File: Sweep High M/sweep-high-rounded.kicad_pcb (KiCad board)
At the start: 2 copper layers, 114.5 x 95.3 mm, 25 parts, among them J2 AudioJack4dpb, SW10 SW_Push, SW11 SW_Push, SW12 SW_Push, SW14 SW_Push, SW15 SW_Push, SW16 SW_Push, SW17 SW_Push, SW18 SW_Push, SW2 SW_Push, SW2 SW_SPDT, SW20 SW_Push, SW21 SW_Push, SW3 SW_Push, SW4 SW_Push, SW5 SW_Push, SW6 SW_Push, SW8 SW_Push, SW9 SW_Push, U1 ProMicro-kbd

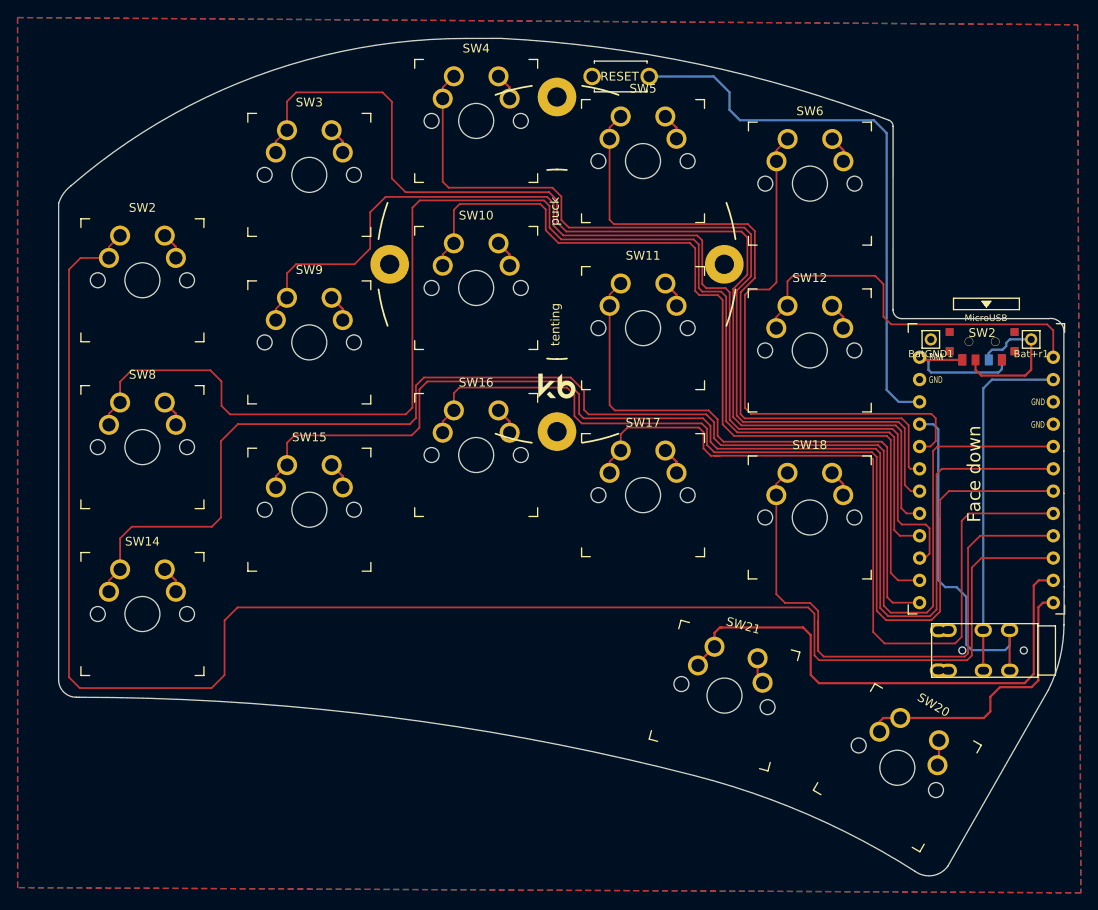
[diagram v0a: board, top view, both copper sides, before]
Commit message: xw
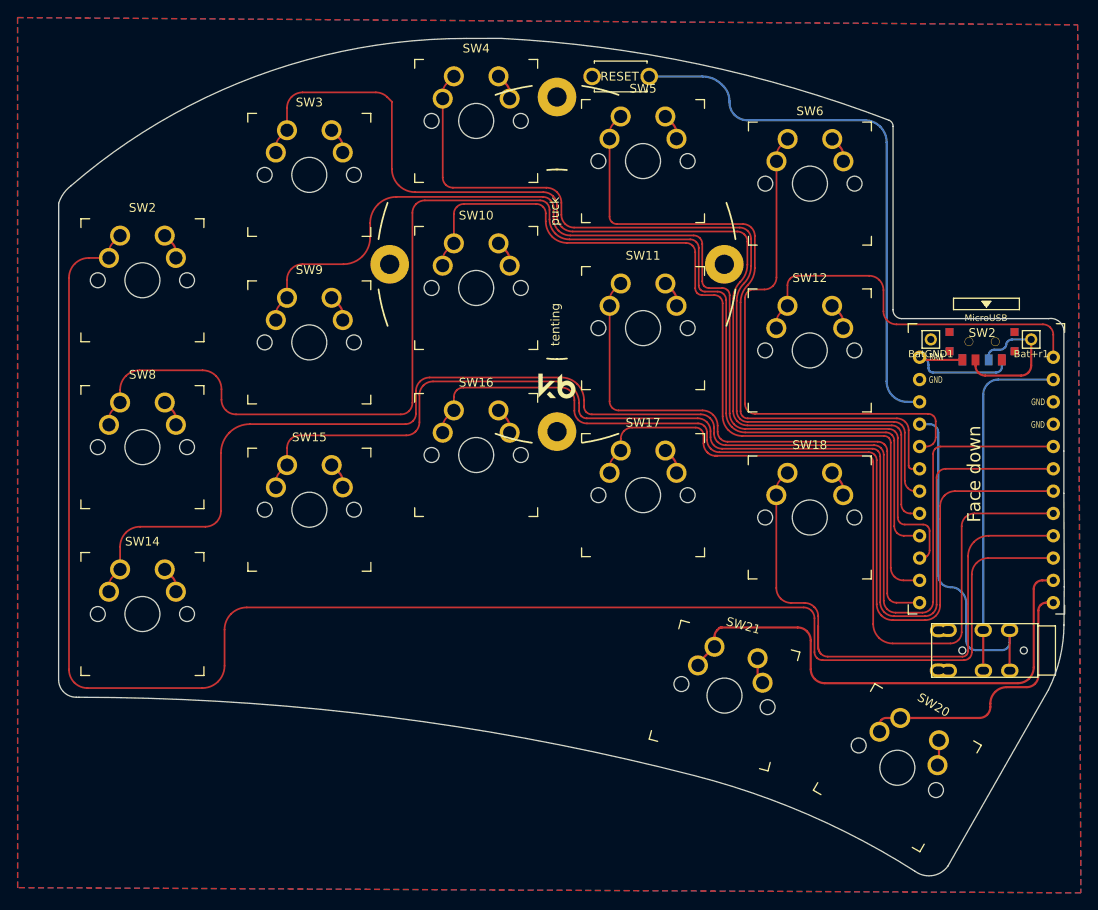
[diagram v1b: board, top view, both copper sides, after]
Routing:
- net gnd: track 53.0 -> 42.4 mm
- net Switch11: track 169.7 -> 165.2 mm
- net Switch6: track 158.8 -> 154.5 mm
- net Switch7: track 122.9 -> 118.7 mm
- net Switch2: track 124.7 -> 120.6 mm
- net Switch13: track 110.8 -> 107.1 mm
- net Switch10: track 44.2 -> 41.2 mm
- net Switch3: track 101.2 -> 98.8 mm
- net Switch12: track 138.0 -> 135.9 mm
- net Switch1: track 190.5 -> 188.5 mm
- net Switch9: track 70.1 -> 68.2 mm
- net Switch14: track 91.7 -> 89.8 mm
- net Switch8: track 99.4 -> 97.5 mm
- net Switch15: track 67.6 -> 66.0 mm
- net Switch4: track 76.6 -> 75.2 mm
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
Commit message: update
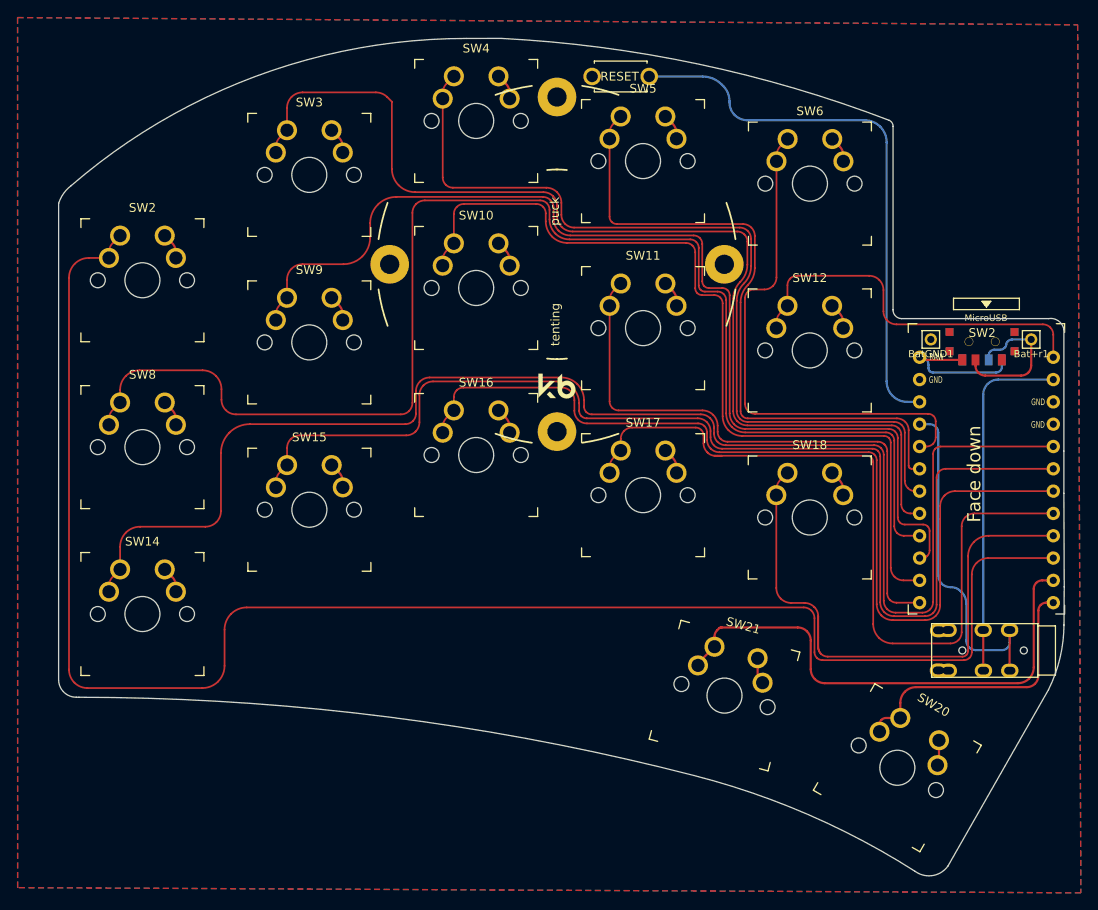
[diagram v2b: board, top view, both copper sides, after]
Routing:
- net gnd: track 42.4 -> 51.9 mm
- net Switch6: track 154.5 -> 156.8 mm
- net Switch10: track 41.2 -> 43.5 mm
- net Switch7: track 118.7 -> 121.0 mm
- net Switch11: track 165.2 -> 167.5 mm
- net Switch2: track 120.6 -> 122.9 mm
- net Switch13: track 107.1 -> 109.4 mm
- net Switch15: track 66.0 -> 67.8 mm
- net Switch17: track 31.0 -> 32.4 mm
- net Switch9: track 68.2 -> 69.4 mm
- net Switch14: track 89.8 -> 91.0 mm
- net Switch3: track 98.8 -> 99.9 mm
- net Switch12: track 135.9 -> 136.5 mm
- net Switch4: track 75.2 -> 75.8 mm
- net Switch5: track 59.6 -> 60.2 mm
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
